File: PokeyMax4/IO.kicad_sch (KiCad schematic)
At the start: 2 parts

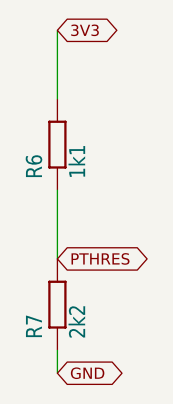
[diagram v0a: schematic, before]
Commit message: Update the v4 board
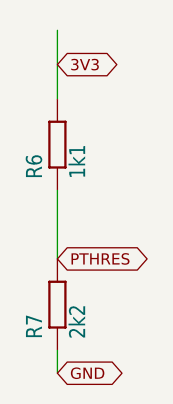
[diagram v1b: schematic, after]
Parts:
- R6: JLCPCB Part # C102771 -> (none); LCSC Part # (none) -> C25860
- R7: JLCPCB Part # C304991 -> (none); LCSC Part # (none) -> C25879
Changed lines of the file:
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@@
+	(wire
+		(pts
+			(xy 144.78 83.82) (xy 144.78 91.44)
+		)
+		(stroke
+			(width 0.1524)
+			(type solid)
+		)
+	)
+	(wire
+		(pts
+			(xy 144.78 119.38) (xy 144.78 121.92)
+		)
+		(stroke
+			(width 0.1524)
+			(type solid)
+		)
+	)
 	(wire
 		(pts
@@
 			(width 0.1524)
 			(type solid)
-		)
-	)
-	(wire
-		(pts
-			(xy 144.78 83.82) (xy 144.78 91.44)
-		)
-		(stroke
-			(width 0.1524)
-			(type solid)
-		)
-	)
-	(wire
-		(pts
-			(xy 144.78 119.38) (xy 144.78 121.92)
-		)
-		(stroke
-			(width 0.1524)
-			(type solid)
-		)
-	)
-	(global_label "3V3"
-		(shape bidirectional)
-		(at 144.78 83.82 0)
-		(fields_autoplaced yes)
-		(effects
-			(font
-				(size 1.2446 1.2446)
-			)
-			(justify left)
-		)
-		(property "Intersheetrefs" "${INTERSHEET_REFS}"
-			(at 152.2316 83.82 0)
-			(effects
-				(font
-					(size 1.27 1.27)
-				)
-				(justify left)
-				(hide yes)
-			)
 		)
 	)
@@
 				(justify left)
 				(hide yes)
+			)
+		)
+	)
+	(global_label "3V3"
+		(shape bidirectional)
+		(at 144.78 87.63 0)
+		(fields_autoplaced yes)
+		(effects
+			(font
+				(size 1.2446 1.2446)
+			)
+			(justify left)
+		)
+		(property "Intersheetrefs" "${INTERSHEET_REFS}"
+			(at 152.2316 87.63 0)
+			(effects
+				(font
+					(size 1.27 1.27)
+				)
+				(justify left)
+				(hide yes)
+			)
+		)
+	)
+	(symbol
+		(lib_id "pokeymax4-eagle-import:R-EU_R0402")
+		(at 144.78 96.52 90)
+		(unit 1)
+		(exclude_from_sim no)
+		(in_bom yes)
+		(on_board yes)
+		(dnp no)
+		(property "Reference" "R6"
+			(at 143.2814 100.33 0)
+			(effects
+				(font
+					(size 1.778 1.5113)
+				)
+				(justify left bottom)
+			)
+		)
+		(property "Value" "1k1"
+			(at 148.082 100.33 0)
+			(effects
+				(font
+					(size 1.778 1.5113)
+				)
+				(justify left bottom)
+			)
+		)
+		(property "Footprint" "pokeymax4:R0402"
+			(at 144.78 96.52 0)
+			(effects
+				(font
+					(size 1.27 1.27)
+				)
+				(hide yes)
+			)
+		)
+		(property "Datasheet" ""
+			(at 144.78 96.52 0)
+			(effects
+				(font
+					(size 1.27 1.27)
+				)
+				(hide yes)
+			)
+		)
+		(property "Description" ""
+			(at 144.78 96.52 0)
+			(effects
+				(font
+					(size 1.27 1.27)
+				)
+				(hide yes)
+			)
+		)
+		(property "LCSC Part #" "C25860"
+			(at 144.78 96.52 0)
+			(effects
+				(font
+					(size 1.27 1.27)
+				)
+				(hide yes)
+			)
+		)
+		(pin "1"
+		)
+		(pin "2"
+		)
+		(instances
+			(project ""
+				(path "/e6275eb3-d183-4a15-8a8c-dffc95cf456c/ffebd24f-75aa-4e21-be2c-b55208e79830"
+					(reference "R6")
+					(unit 1)
+				)
 			)
 		)
@@
 			)
 		)
-		(property "JLCPCB Position Offset" ""
-			(at 144.78 114.3 0)
-			(effects
-				(font
-					(size 1.27 1.27)
-				)
-				(hide yes)
-			)
-		)
-		(property "JLCPCB Rotation Offset" ""
-			(at 144.78 114.3 0)
-			(effects
-				(font
-					(size 1.27 1.27)
-				)
-				(hide yes)
-			)
-		)
-		(property "JLCPCB Part #" "C304991"
-			(at 144.78 114.3 0)
-			(effects
-				(font
-					(size 1.27 1.27)
-				)
-				(hide yes)
-			)
+		(property "LCSC Part #" " C25879"
+			(at 144.78 114.3 0)
+			(effects
+				(font
+					(size 1.27 1.27)
+				)
+				(hide yes)
+			)
+		)
+		(pin "1"
 		)
 		(pin "2"
 		)
-		(pin "1"
-		)
 		(instances
-			(project "pokeymax4"
-				(path "/87a5706b-9c3d-497f-99bc-f4f71751dafe/b931f0b5-7d10-4325-a72c-13a8b4fa7819"
+			(project ""
+				(path "/e6275eb3-d183-4a15-8a8c-dffc95cf456c/ffebd24f-75aa-4e21-be2c-b55208e79830"
 					(reference "R7")
 					(unit 1)
 				)
-			)
-		)
-	)
-	(symbol
-		(lib_id "pokeymax4-eagle-import:R-EU_R0402")
-		(at 144.78 96.52 90)
-		(unit 1)
-		(exclude_from_sim no)
-		(in_bom yes)
-		(on_board yes)
-		(dnp no)
-		(property "Reference" "R6"
-			(at 143.2814 100.33 0)
-			(effects
-				(font
-					(size 1.778 1.5113)
-				)
-				(justify left bottom)
-			)
-		)
-		(property "Value" "1k1"
-			(at 148.082 100.33 0)
-			(effects
-				(font
-					(size 1.778 1.5113)
-				)
-				(justify left bottom)
-			)
-		)
-		(property "Footprint" "pokeymax4:R0402"
-			(at 144.78 96.52 0)
-			(effects
-				(font
-					(size 1.27 1.27)
-				)
-				(hide yes)
-			)
-		)
-		(property "Datasheet" ""
-			(at 144.78 96.52 0)
-			(effects
-				(font
-					(size 1.27 1.27)
-				)
-				(hide yes)
-			)
-		)
-		(property "Description" ""
-			(at 144.78 96.52 0)
-			(effects
-				(font
-					(size 1.27 1.27)
-				)
-				(hide yes)
-			)
-		)
-		(property "JLCPCB Position Offset" ""
-			(at 144.78 96.52 0)
-			(effects
-				(font
-					(size 1.27 1.27)
-				)
-				(hide yes)
-			)
-		)
-		(property "JLCPCB Rotation Offset" ""
-			(at 144.78 96.52 0)
-			(effects
-				(font
-					(size 1.27 1.27)
-				)
-				(hide yes)
-			)
-		)
-		(property "JLCPCB Part #" "C102771"
-			(at 144.78 96.52 0)
-			(effects
-				(font
-					(size 1.27 1.27)
-				)
-				(hide yes)
-			)
-		)
-		(pin "1"
-		)
-		(pin "2"
-		)
-		(instances
-			(project "pokeymax4"
-				(path "/87a5706b-9c3d-497f-99bc-f4f71751dafe/b931f0b5-7d10-4325-a72c-13a8b4fa7819"
-					(reference "R6")
-					(unit 1)
-				)
